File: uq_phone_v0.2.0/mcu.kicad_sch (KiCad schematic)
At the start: 34 parts, among them J6 Conn_ARM_SWD_TagConnect_TC2030, J7 559092474, J9 559092474, Q1 MMBT3904LP-7, Q2 MMBT3904LP-7, U16 TXB0108YZPR2, U5 TCA9509MRVHR, U6 STM32H733VGHx, U7 TXB0108YZPR2

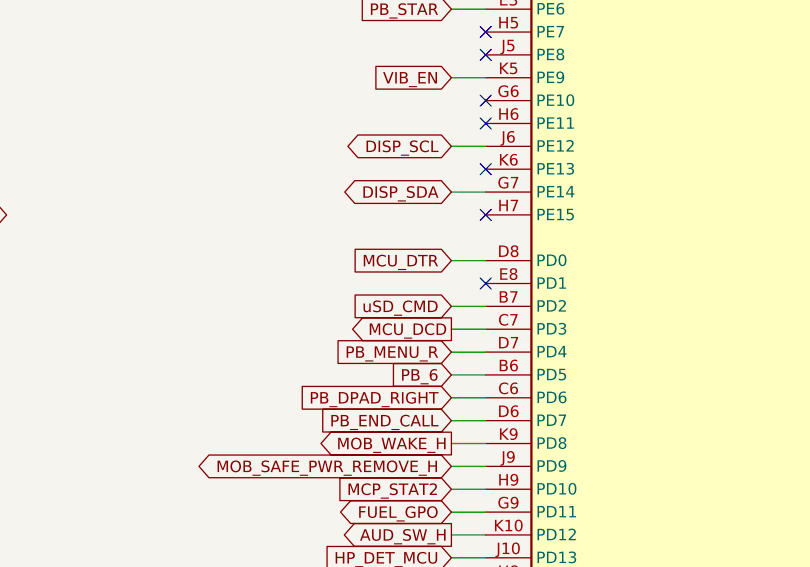
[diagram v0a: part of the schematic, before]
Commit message: DRC and routing fixing
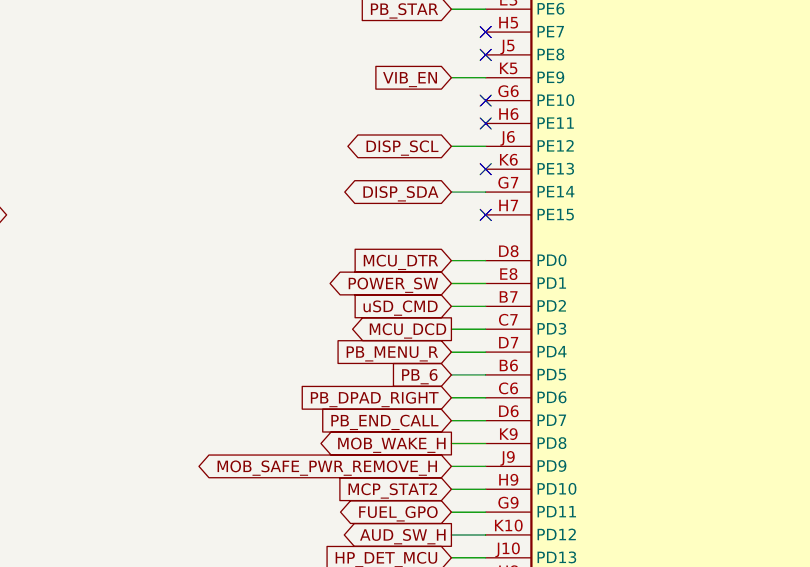
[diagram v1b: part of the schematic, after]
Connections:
- net POWER_SW: now reaches U6.E8 (PD1)
- no-connect marks 18 -> 17
